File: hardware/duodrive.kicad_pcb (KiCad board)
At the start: 2 copper layers, 49 x 75 mm, 110 parts, among them J2 Conn_02x08_Odd_Even, J3 Conn_01x03, J4 Conn_01x04, J5 Conn_01x04, J6 Conn_01x06, J7 Conn_01x04, J8 Conn_01x04, Q1 AOD4184, Q2 AOD4184, Q3 AOD4184, Q4 AOD4184, Q5 AOD4184, Q6 AOD4184, Q7 AOD4184, Q8 AOD4184, U10 MIC5219-3.3YM5, U2 IR2011, U3 TPS62173DSG, U4 STM32G431RBTx, U5 IR2011, U6 IR2011, U7 IR2011, U8 TPS62933, U9 TJA1042T, Y1 Resonator

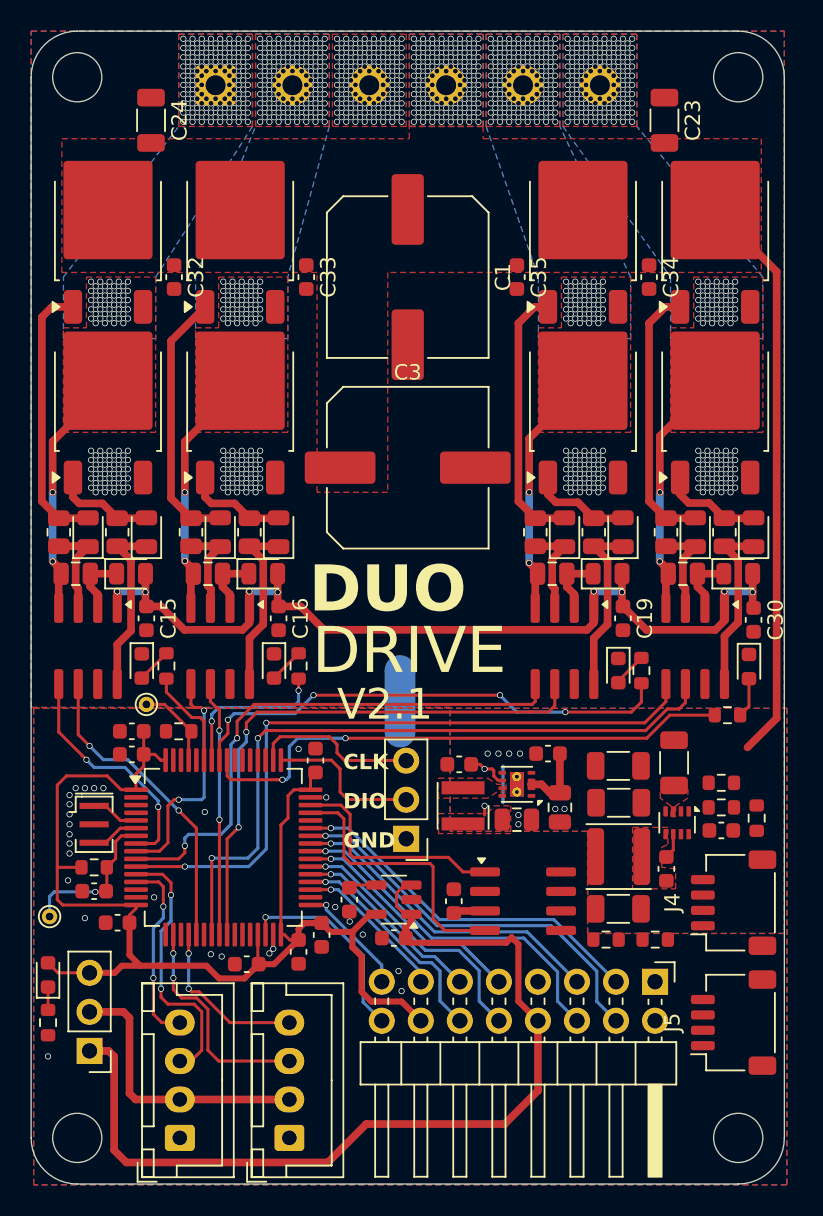
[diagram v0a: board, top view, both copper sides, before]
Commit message: finish and polishing
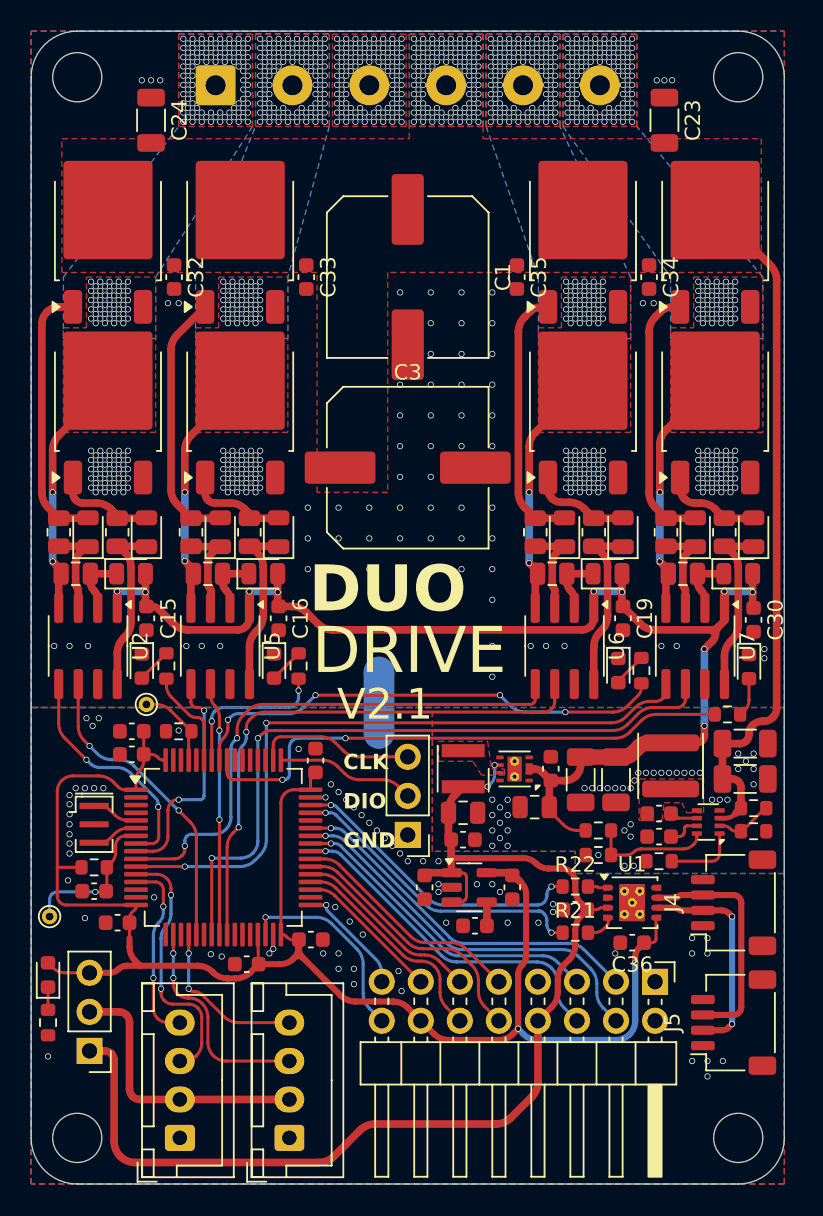
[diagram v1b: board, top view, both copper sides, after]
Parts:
- removed U9: TJA1042T, 1_NoOutline:SOIC-8_3.9x4.9mm_P1.27mm
- added C36: 100nF, Capacitor_SMD:C_0603_1608Metric, F.Cu at (129.1, 109.3)
- added R21: 47R, Resistor_SMD:R_0603_1608Metric, F.Cu at (125.4, 108.7)
- added R22: 47R, Resistor_SMD:R_0603_1608Metric, F.Cu at (125.4, 105.7)
- added U1: TCAN1044V, Package_SON:Texas_S-PVSON-N8_ThermalVias, F.Cu at (129.1, 106.7)
- C1, C3: value 680uF -> 470uF
- J3: value Conn_01x03 -> SWD
- J4: value Conn_01x04 -> CAN_IN
- J5: value Conn_01x04 -> CAN_OUT
- J6: value Conn_01x06 -> POWER
- J7: value Conn_01x04 -> ENCODER1
- J8: value Conn_01x04 -> ENCODER2
- U2, U5, U6, U7: footprint 1_NoOutline:SOIC-8_3.9x4.9mm_P1.27mm -> Package_SO:SOIC-8_3.9x4.9mm_P1.27mm
- moved C12 12.8 mm to (121.3, 105.7)
- moved C28 8.40 mm to (128.1, 98.7), turned to 90 degrees
- moved C27 8.38 mm to (136.4, 96.3), turned to 180 degrees
- moved C26 8.35 mm to (118.9, 108.2), turned to 180 degrees
- moved C13 7.92 mm to (125.4, 107.2), turned to 180 degrees
- moved R4 7.12 mm to (126.9, 102.0)
- moved L1 6.80 mm to (131.6, 97.8), turned to 90 degrees
- moved R6 6.63 mm to (126.9, 103.6), turned to 0 degrees
- moved R11 5.35 mm to (130.8, 104.0), turned to 0 degrees
- moved U10 4.96 mm to (118.5, 105.7), turned to 0 degrees
- moved C42 4.91 mm to (118.1, 102.6), turned to 0 degrees
- moved C18 4.74 mm to (136.4, 98.7), turned to 180 degrees
- moved C25 4.07 mm to (130.8, 102.4), turned to 0 degrees
- moved C10 3.86 mm to (115.6, 105.7), turned to -90 degrees
- moved C6 3.63 mm to (130.8, 100.9), turned to 0 degrees
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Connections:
- J4 pad 2: unconnected-(J4-Pin_2-Pad2) -> CAN_L
- J4 pad 3: unconnected-(J4-Pin_3-Pad3) -> CAN_H
- J5 pad 2: unconnected-(J5-Pin_2-Pad2) -> CAN_L
- J5 pad 3: unconnected-(J5-Pin_3-Pad3) -> CAN_H
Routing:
- net +3.3V: track 78.8 -> 108.7 mm, vias 0 -> 2
- net +10V: track 64.2 -> 85.1 mm, vias 8 -> 10
- net CAN_H: track 0.00 -> 15.4 mm
- net CAN_L: track 0.00 -> 14.0 mm, vias 0 -> 2
- net +5V: track 65.8 -> 77.1 mm
- net VDC: track 37.4 -> 45.5 mm, vias 131 -> 106
- net Net-(U8-FB): track 0.00 -> 7.92 mm
- net CANTX: track 14.7 -> 19.7 mm, vias 0 -> 2
- net Net-(U8-RT): track 0.00 -> 4.70 mm
- net Net-(U8-EN): track 0.00 -> 3.73 mm
- net (no net): track 2.40 -> 0.00 mm, vias 1 -> 0
- net Net-(U8-SS): track 0.00 -> 2.16 mm
- net CANRX: track 18.0 -> 19.9 mm, vias 0 -> 2
- net Net-(U1-RXD): track 0.00 -> 1.91 mm
- net Net-(U1-TXD): track 0.00 -> 1.14 mm
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- removed copper zone on F.Cu, net +5V
